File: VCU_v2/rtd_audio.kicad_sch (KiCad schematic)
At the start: 52 parts, among them U12 TPA3116D2QDADRQ1, U13 PCM5102APWR

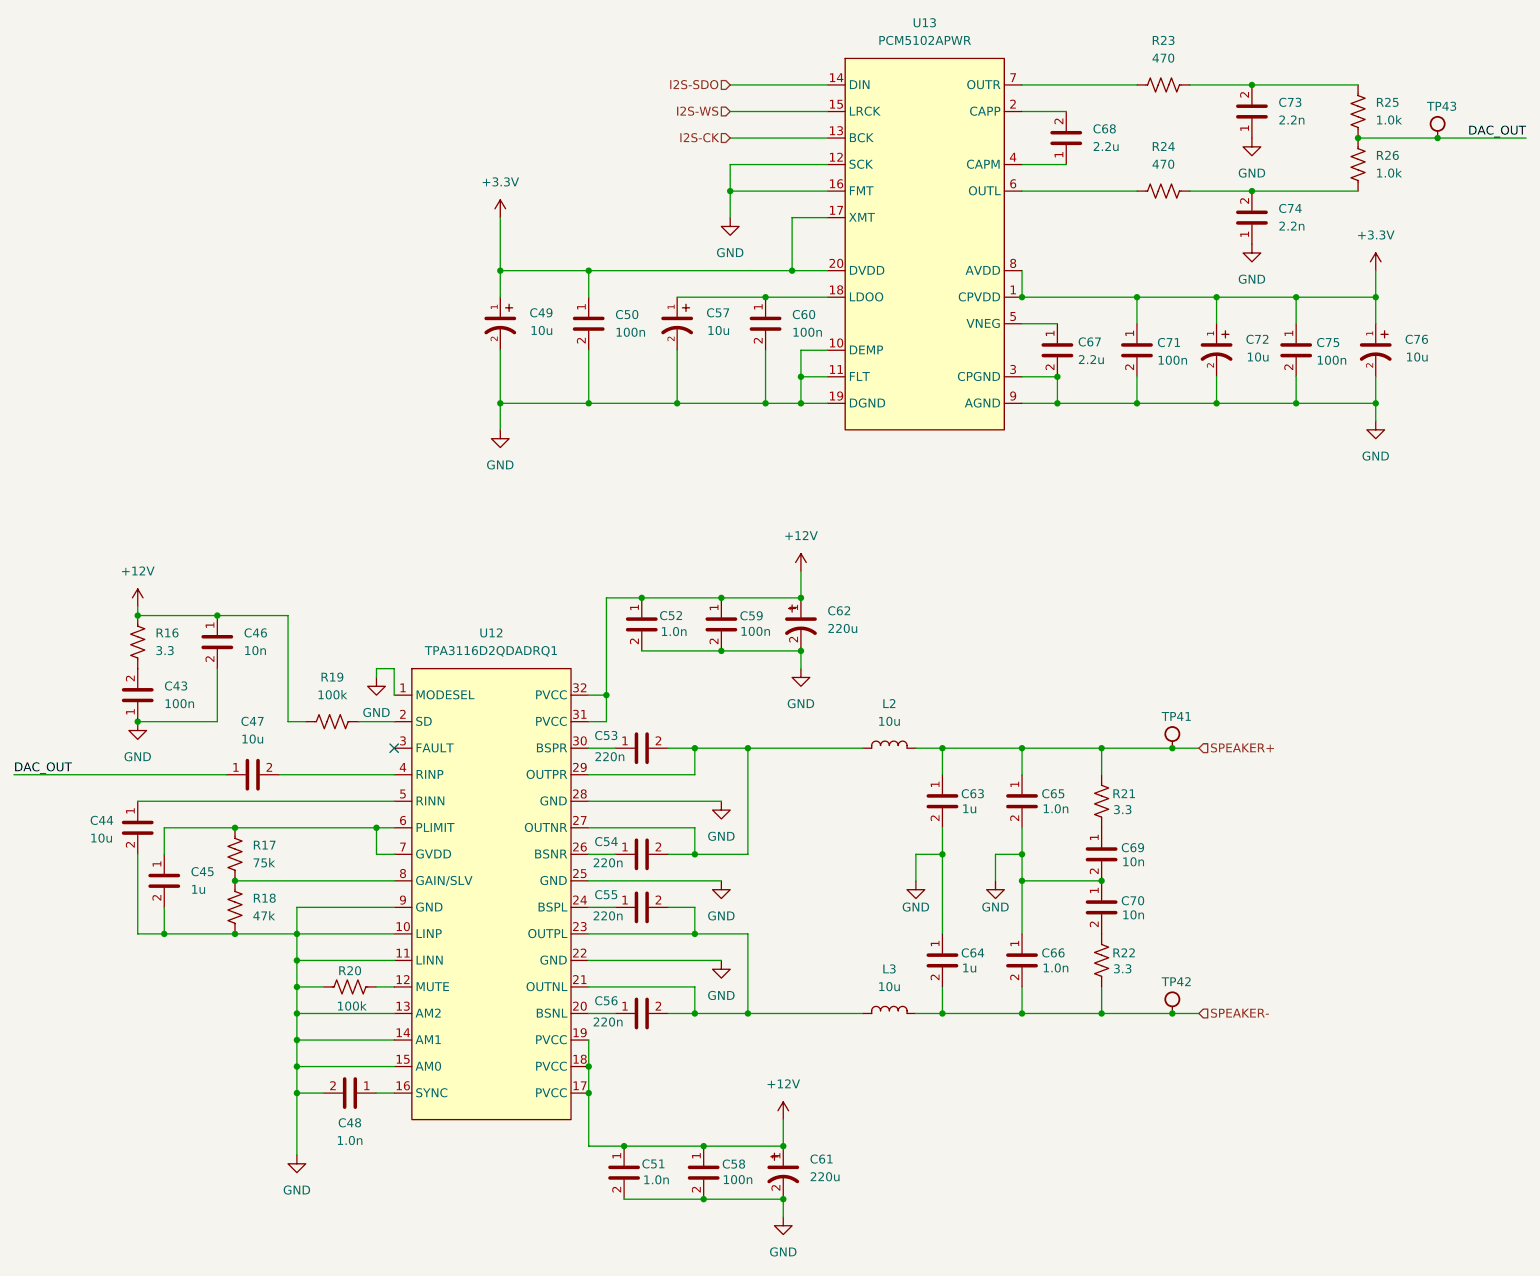
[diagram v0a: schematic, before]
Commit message: placements friggin 80% friggin done shoutout epstein
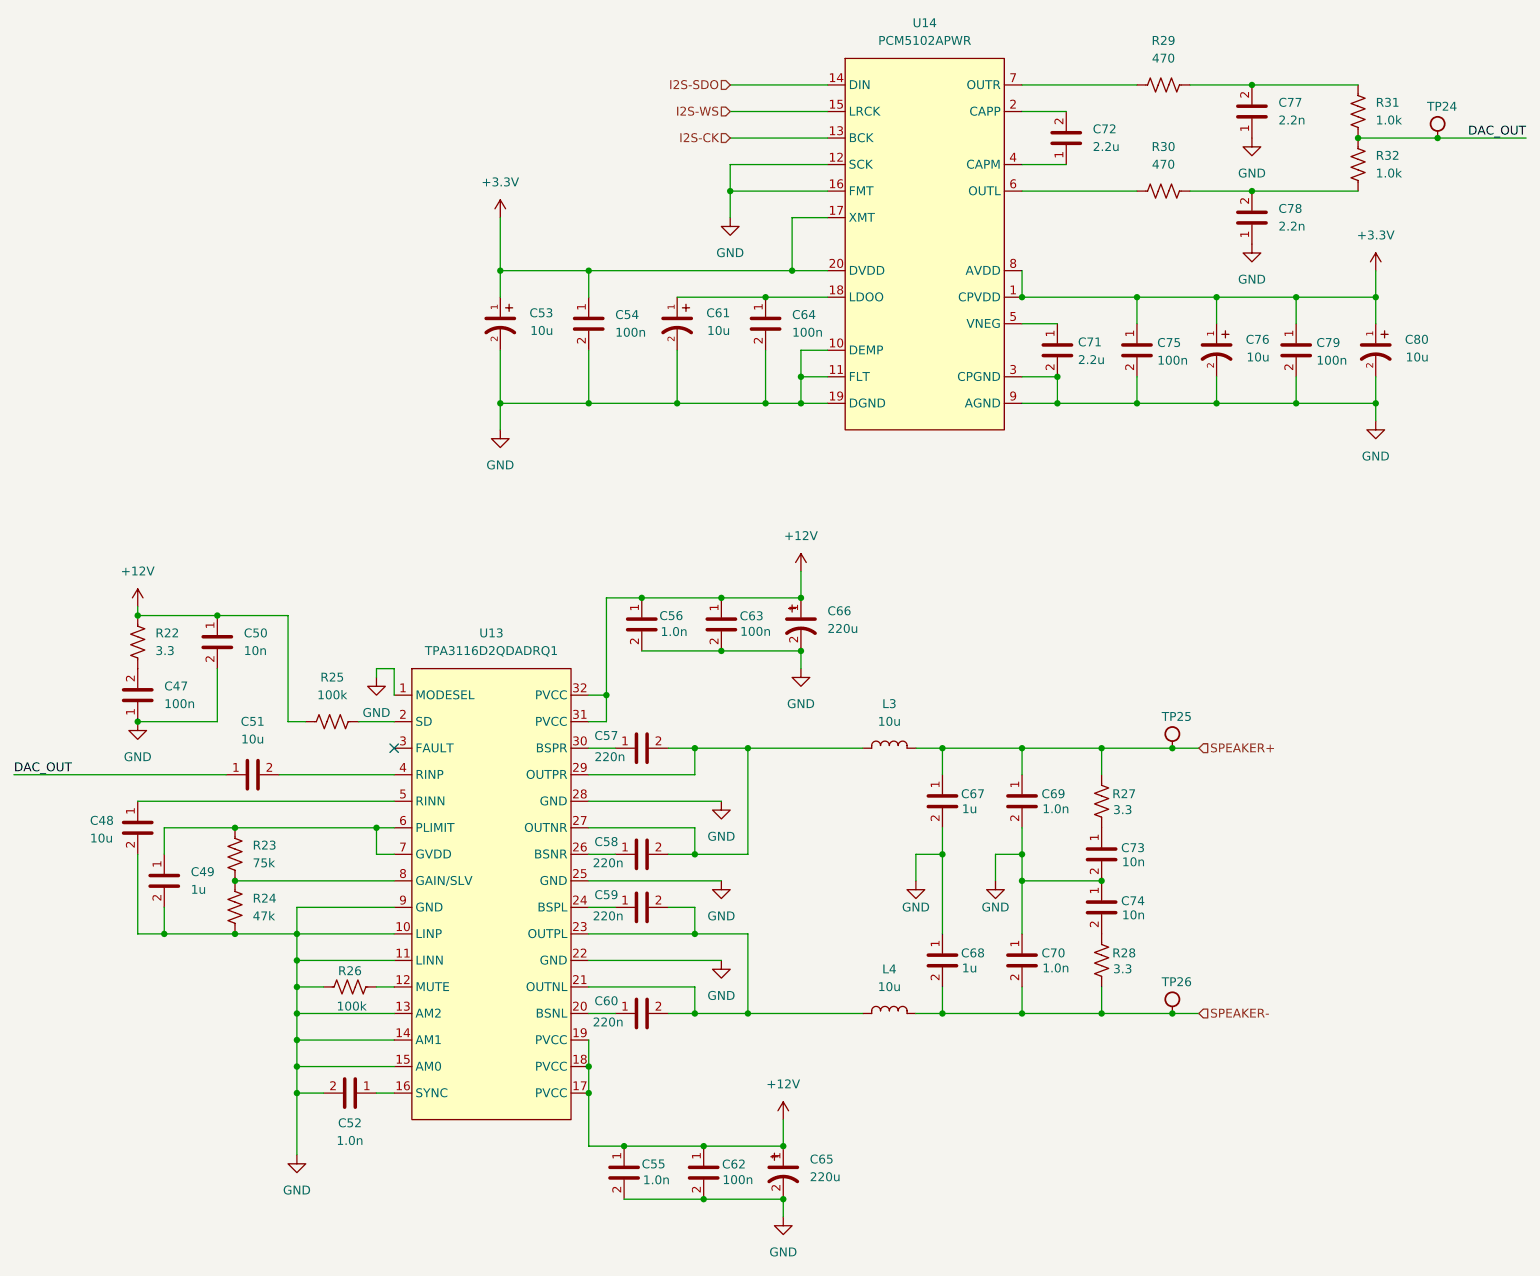
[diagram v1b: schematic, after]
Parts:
- renumbered C43 to C47, C44 to C48, C45 to C49, C46 to C50, C47 to C51, C48 to C52, C49 to C53, C50 to C54, C51 to C55, C52 to C56, C53 to C57, C54 to C58, C55 to C59, C56 to C60, C57 to C61, C58 to C62, C59 to C63, C60 to C64, C61 to C65, C62 to C66, C63 to C67, C64 to C68, C65 to C69, C66 to C70, C67 to C71, C68 to C72, C69 to C73, C70 to C74, C71 to C75, C72 to C76, C73 to C77, C74 to C78, C75 to C79, C76 to C80, L2 to L3, L3 to L4, R16 to R22, R17 to R23, R18 to R24, R19 to R25, R20 to R26, R21 to R27, R22 to R28, R23 to R29, R24 to R30, R25 to R31, R26 to R32, TP43 to TP24, TP41 to TP25, TP42 to TP26, U12 to U13, U13 to U14

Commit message: vcu v2 schematics done
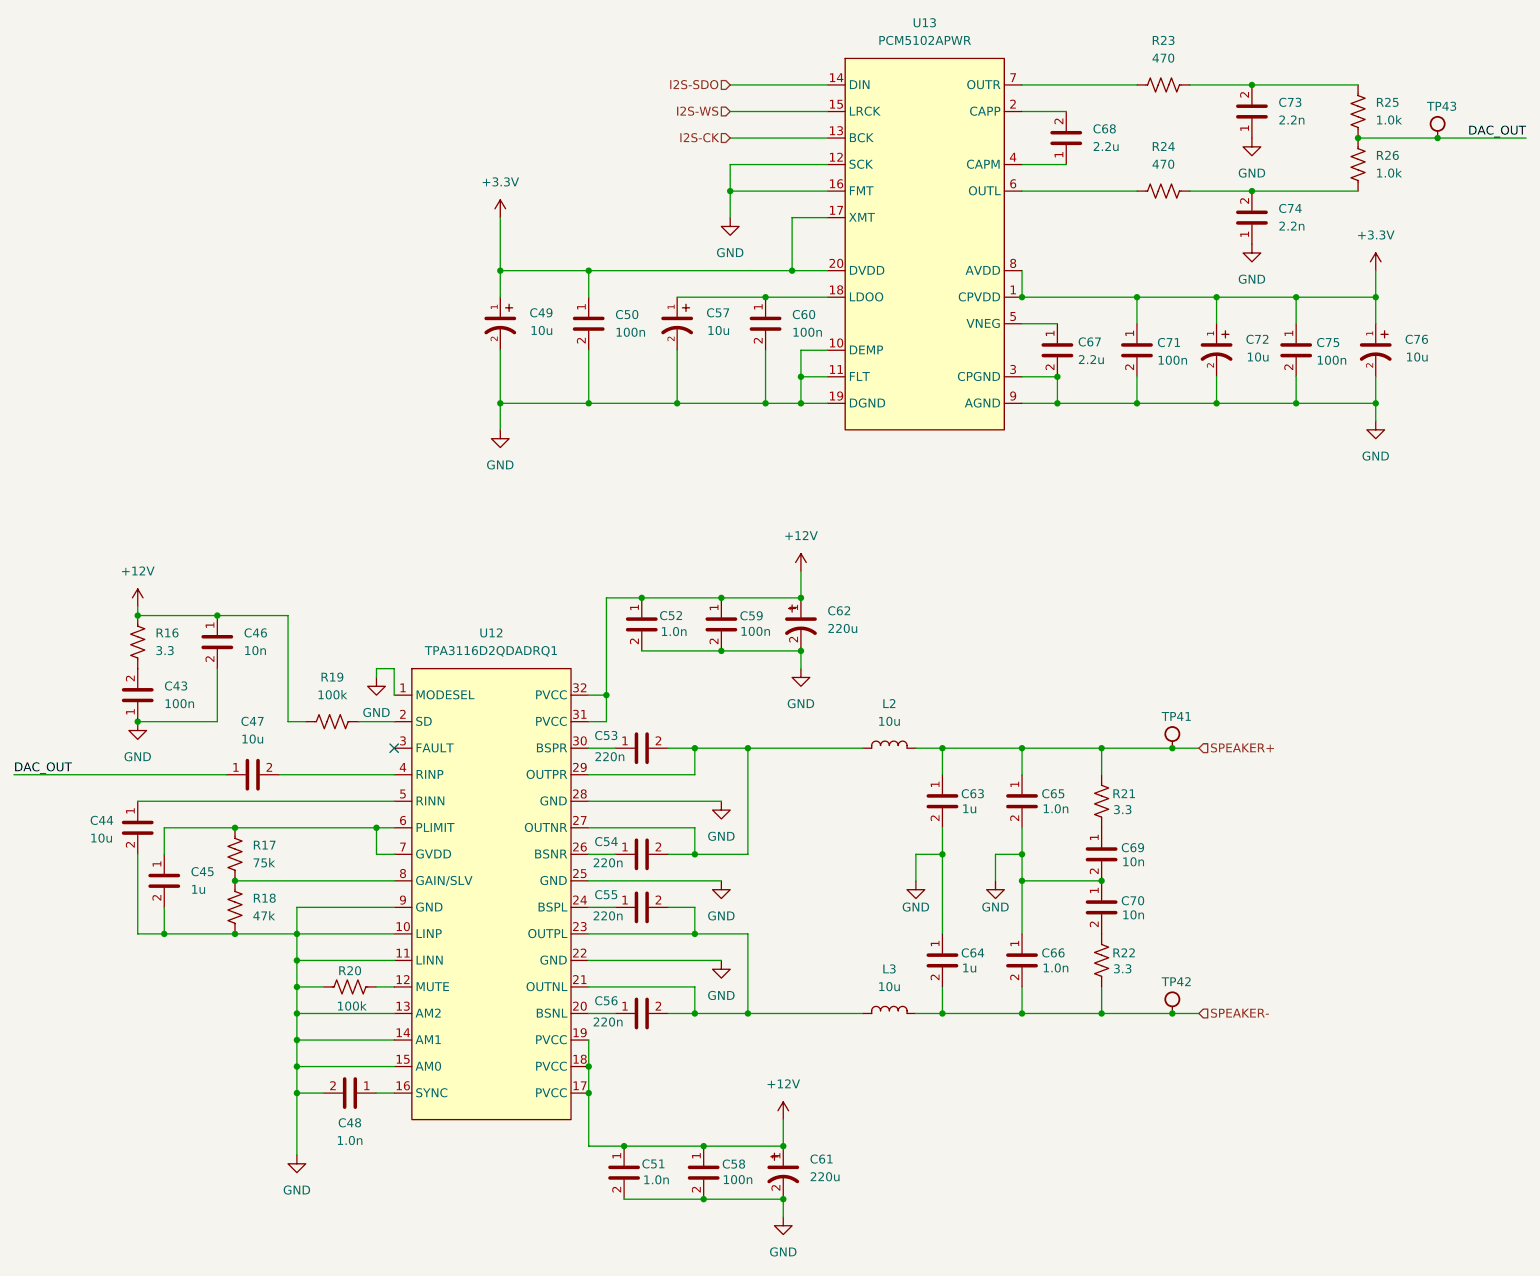
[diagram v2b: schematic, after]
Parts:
- renumbered C47 to C43, C48 to C44, C49 to C45, C50 to C46, C51 to C47, C52 to C48, C53 to C49, C54 to C50, C55 to C51, C56 to C52, C57 to C53, C58 to C54, C59 to C55, C60 to C56, C61 to C57, C62 to C58, C63 to C59, C64 to C60, C65 to C61, C66 to C62, C67 to C63, C68 to C64, C69 to C65, C70 to C66, C71 to C67, C72 to C68, C73 to C69, C74 to C70, C75 to C71, C76 to C72, C77 to C73, C78 to C74, C79 to C75, C80 to C76, L3 to L2, L4 to L3, R22 to R16, R23 to R17, R24 to R18, R25 to R19, R26 to R20, R27 to R21, R28 to R22, R29 to R23, R30 to R24, R31 to R25, R32 to R26, TP25 to TP41, TP26 to TP42, TP24 to TP43, U13 to U12, U14 to U13
